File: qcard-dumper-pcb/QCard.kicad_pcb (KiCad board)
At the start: 2 copper layers, 2 parts, among them J1 Conn_02x18_Top_Bottom, U1 AT27C040-70PU

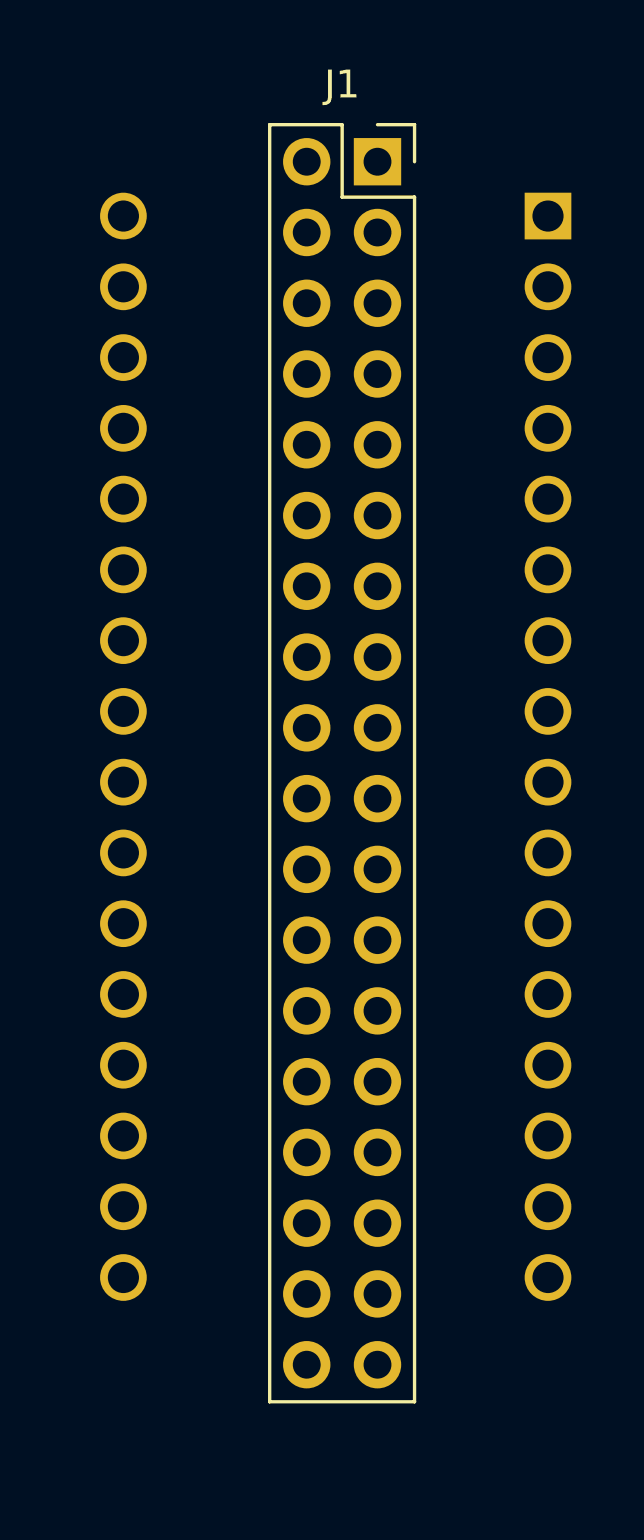
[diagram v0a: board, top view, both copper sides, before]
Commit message: Dumper v1
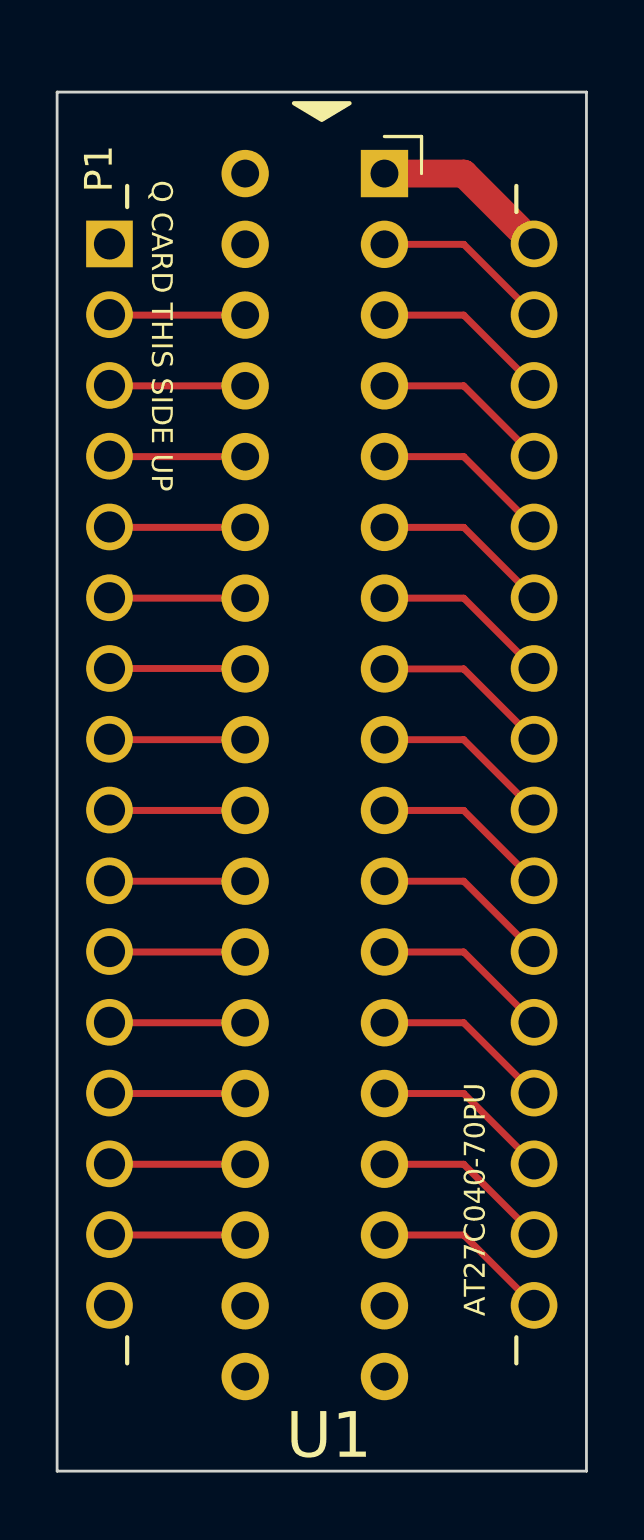
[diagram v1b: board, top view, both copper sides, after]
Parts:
- J1: value Conn_02x18_Top_Bottom -> Conn_02x18_Odd_Even
- U1: moved to F.Cu
- moved U1 14.8 mm to (101.1, 93.5), turned to 0 degrees
- moved J1 0.49 mm to (95.8, 52.9)
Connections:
- J1 pad 1: /GND -> /VCC
- J1 pad 10: /A3 -> /A12
- J1 pad 11: /A2 -> /A8
- J1 pad 12: /A1 -> /A7
- J1 pad 13: /A0 -> /A9
- J1 pad 14: /D0 -> /A6
- J1 pad 15: /D1 -> /A11
- J1 pad 16: /D2 -> /A5
- J1 pad 17: /GND -> /OE
- J1 pad 18: unconnected-(J1-Pad18) -> /A4
- J1 pad 19: /VCC -> /A10
- J1 pad 20: /A18 -> /A3
- J1 pad 21: /A17 -> /CE
- J1 pad 22: /A14 -> /A2
- J1 pad 23: /A13 -> /D7
- J1 pad 24: /A8 -> /A1
- J1 pad 25: /A9 -> /D6
- J1 pad 26: /OE -> /A0
- J1 pad 27: /A10 -> /D5
- J1 pad 28: /CE -> /D0
- J1 pad 29: /D7 -> /D4
- J1 pad 3: /A16 -> /A18
- J1 pad 30: /D6 -> /D1
- J1 pad 31: /D5 -> /D3
- J1 pad 32: /D4 -> /D2
- J1 pad 33: /D3 -> /GND
- J1 pad 34: /D2 -> /GND
- J1 pad 36: /GND -> unconnected-(J1-Pad36)
- J1 pad 4: /A15 -> /GND
- J1 pad 5: /A12 -> /A17
- J1 pad 6: /A7 -> /A16
- J1 pad 7: /A6 -> /A14
- J1 pad 8: /A5 -> /A15
- J1 pad 9: /A4 -> /A13
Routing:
- net /VCC: track 0.00 -> 6.42 mm
- net /D7: track 0.00 -> 6.42 mm
- net /D6: track 0.00 -> 6.42 mm
- net /D5: track 0.00 -> 6.42 mm
- net /D4: track 0.00 -> 6.42 mm
- net /A8: track 0.00 -> 6.42 mm
- net /A11: track 0.00 -> 6.42 mm
- net /A10: track 0.00 -> 6.42 mm
- net /A18: track 0.00 -> 6.42 mm
- net /A17: track 0.00 -> 6.42 mm
- net /A14: track 0.00 -> 6.42 mm
- net /A13: track 0.00 -> 6.42 mm
- net /OE: track 0.00 -> 6.42 mm
- net /D3: track 0.00 -> 6.42 mm
- net /CE: track 0.00 -> 6.42 mm
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- added copper zone on B.Cu, net /GND
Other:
- board outline added: 19 x 49.5 mm
- board text added: "P1"
- board text added: "Q CARD THIS SIDE UP"
